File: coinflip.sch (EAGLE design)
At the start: 17 parts, among them IC1 LM358N, IC2 4027N, T1 2N3904, T2 2N3904

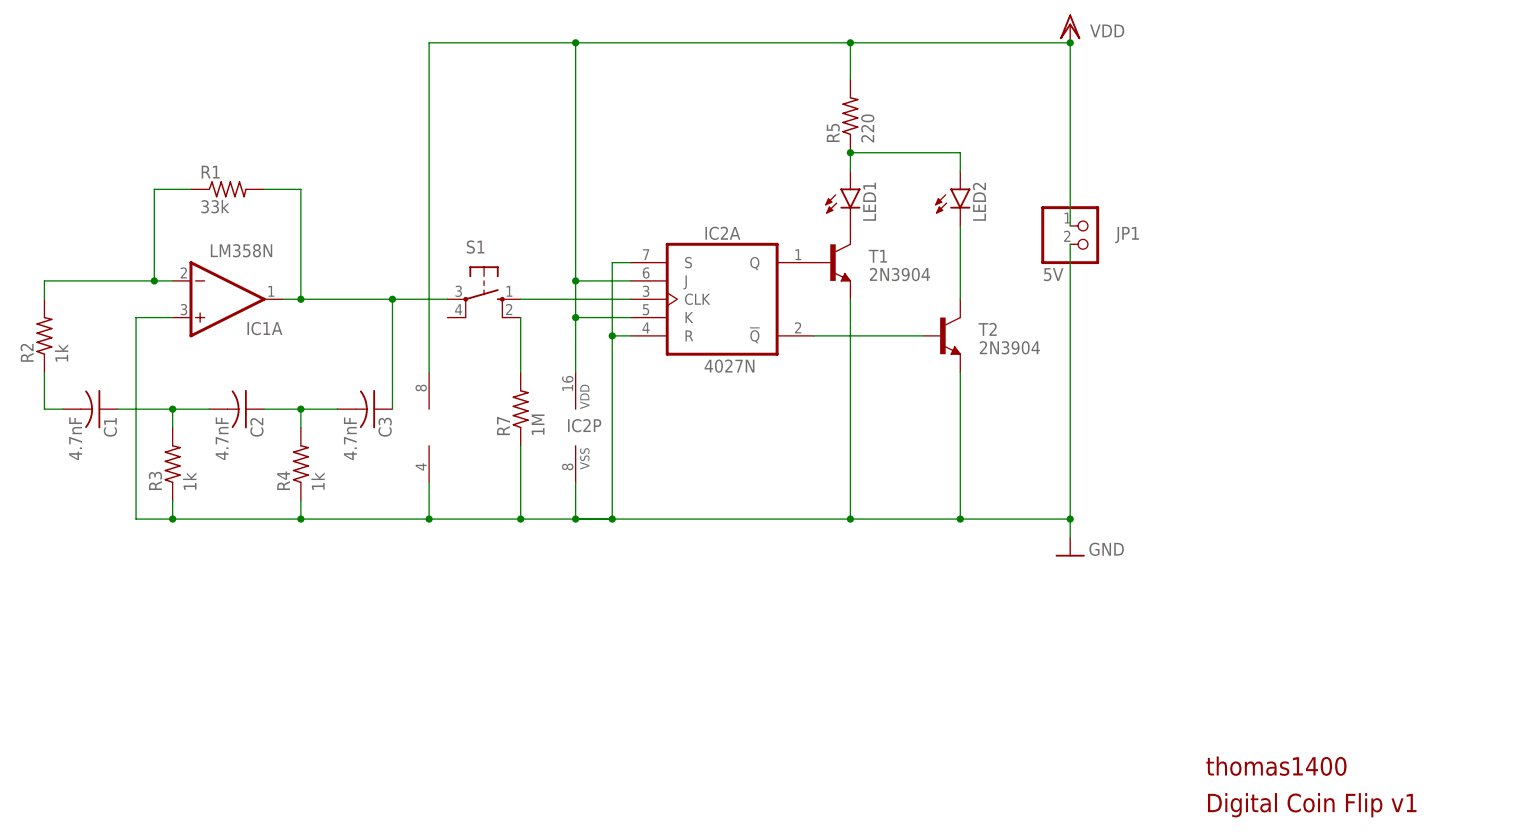
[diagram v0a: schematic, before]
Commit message: Version 2.0 commit
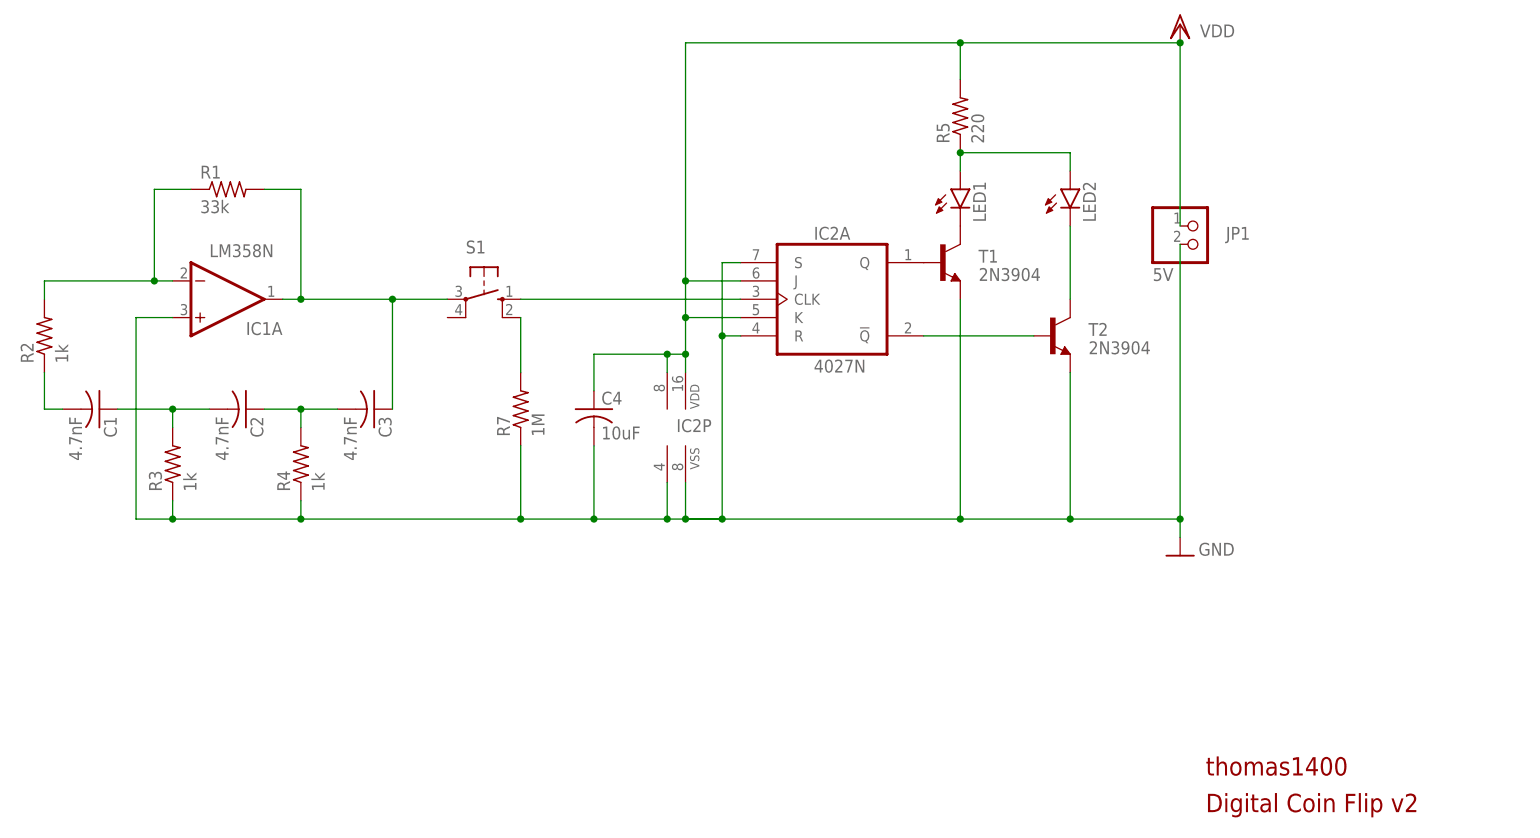
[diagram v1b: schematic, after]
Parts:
- added C4: 10uF, rcl:C-US025-024X044
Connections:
- net GND: now also C4.2
- net VDD: now also C4.1
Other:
- note added: "Digital Coin Flip v2"
- note removed: "Digital Coin Flip v1"
- moved on the sheet: IC2A, IC2P, JP1, LED1, LED2, R5, T1, T2
